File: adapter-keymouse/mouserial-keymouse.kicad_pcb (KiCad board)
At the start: 2 copper layers, 42.5 x 39.4 mm, 13 parts, among them J1 Mouserial, J2 Mouse, J3 Keybd

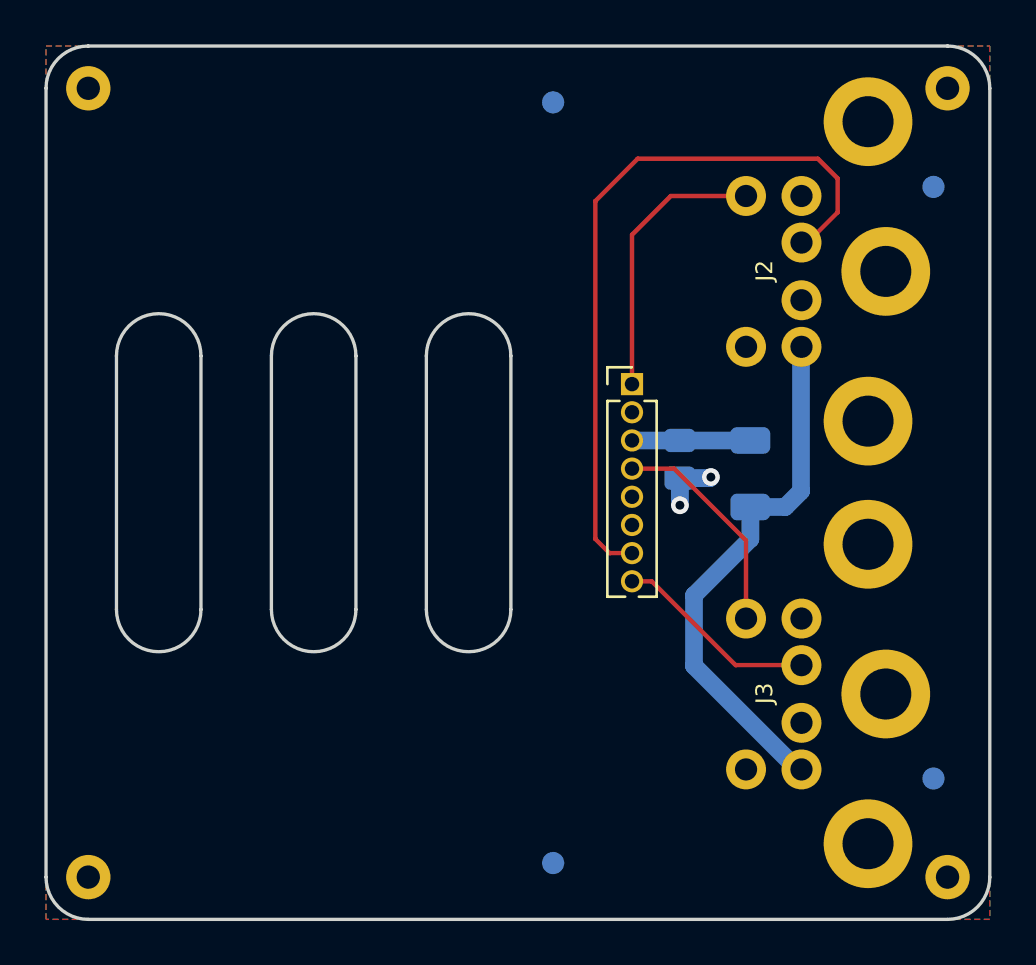
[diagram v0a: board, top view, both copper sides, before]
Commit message: Adapter stuff, avr
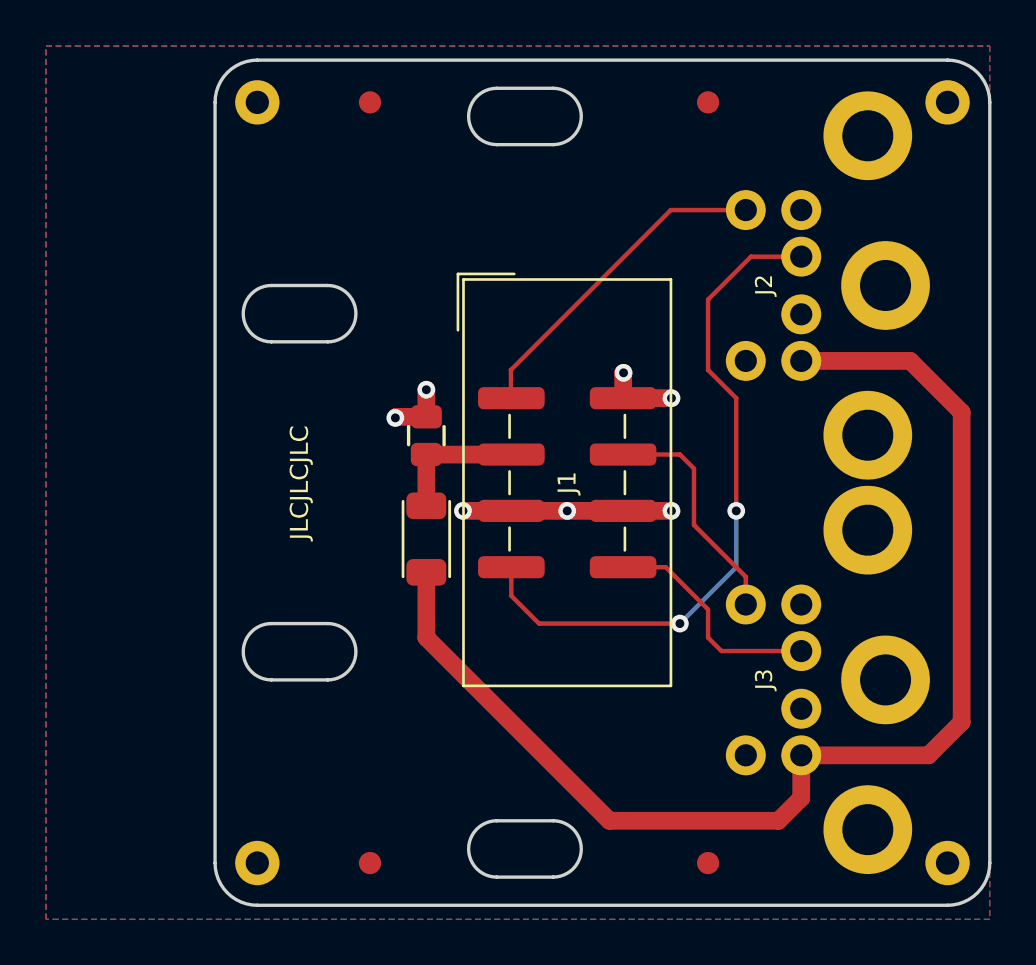
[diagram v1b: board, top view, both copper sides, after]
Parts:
- C1, F1, FID1, FID2, FID3, FID4: moved to F.Cu
- J1: footprint Connector_PinHeader_1.27mm:PinHeader_1x08_P1.27mm_Vertical -> stdpads:IDC_SMD_2x04_P2.54mm_Vertical
- moved FID1 35.3 mm to (151.1, 101.6)
- moved FID2 35.3 mm to (151.1, 67.3), turned to 180 degrees
- moved F1 14.9 mm to (153.7, 87.0)
- moved C1 11.5 mm to (153.7, 82.3), turned to 90 degrees
- moved FID4 10.9 mm to (166.4, 67.3), turned to 180 degrees
- moved FID3 10.9 mm to (166.4, 101.6), turned to 180 degrees
- moved H1 7.65 mm to (146.1, 67.3)
- moved H2 7.65 mm to (146.1, 101.6)
- moved J1 5.32 mm to (160.0, 84.5)
- moved J3 0.64 mm to (179.1, 93.3)
- moved J2 0.64 mm to (179.1, 75.6)
- moved H3 0.64 mm to (177.2, 101.6)
- moved H4 0.64 mm to (177.2, 67.3)
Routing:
- net +5V: track 23.7 -> 55.6 mm
- net GND: track 2.64 -> 15.4 mm, vias 2 -> 7
- net /MDat: track 33.0 -> 30.6 mm, vias 0 -> 2
- net /MClk: track 12.6 -> 14.9 mm
- net /KDat: track 9.21 -> 10.3 mm
- net Net-(C1-Pad1): track 5.33 -> 6.14 mm
- net /KClk: track 10.0 -> 10.6 mm
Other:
- board size 42.5 x 39.4 mm -> 34.9 x 38.1 mm
